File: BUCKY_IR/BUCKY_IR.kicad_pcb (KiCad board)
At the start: 2 copper layers, 189.9 x 157.6 mm, 37 parts, among them J1 SERIAL_CONN, J2 CAN_CONN_UP, J3 CAN_CONN_DOWN, U1 TSSP96038TR, U10 TSSP96038TR, U11 TSSP96038TR, U12 TSSP96038TR, U13 TSSP96038TR, U14 TSSP96038TR, U15 TSSP96038TR, U16 TSSP96038TR, U17 SN65HVD230, U18 ESP32-WROOM-32U, U19 AMS1117-5.0, U2 TSSP96038TR, U3 TSSP96038TR, U4 TSSP96038TR, U5 TSSP96038TR, U6 TSSP96038TR, U7 TSSP96038TR, U8 TSSP96038TR, U9 TSSP96038TR

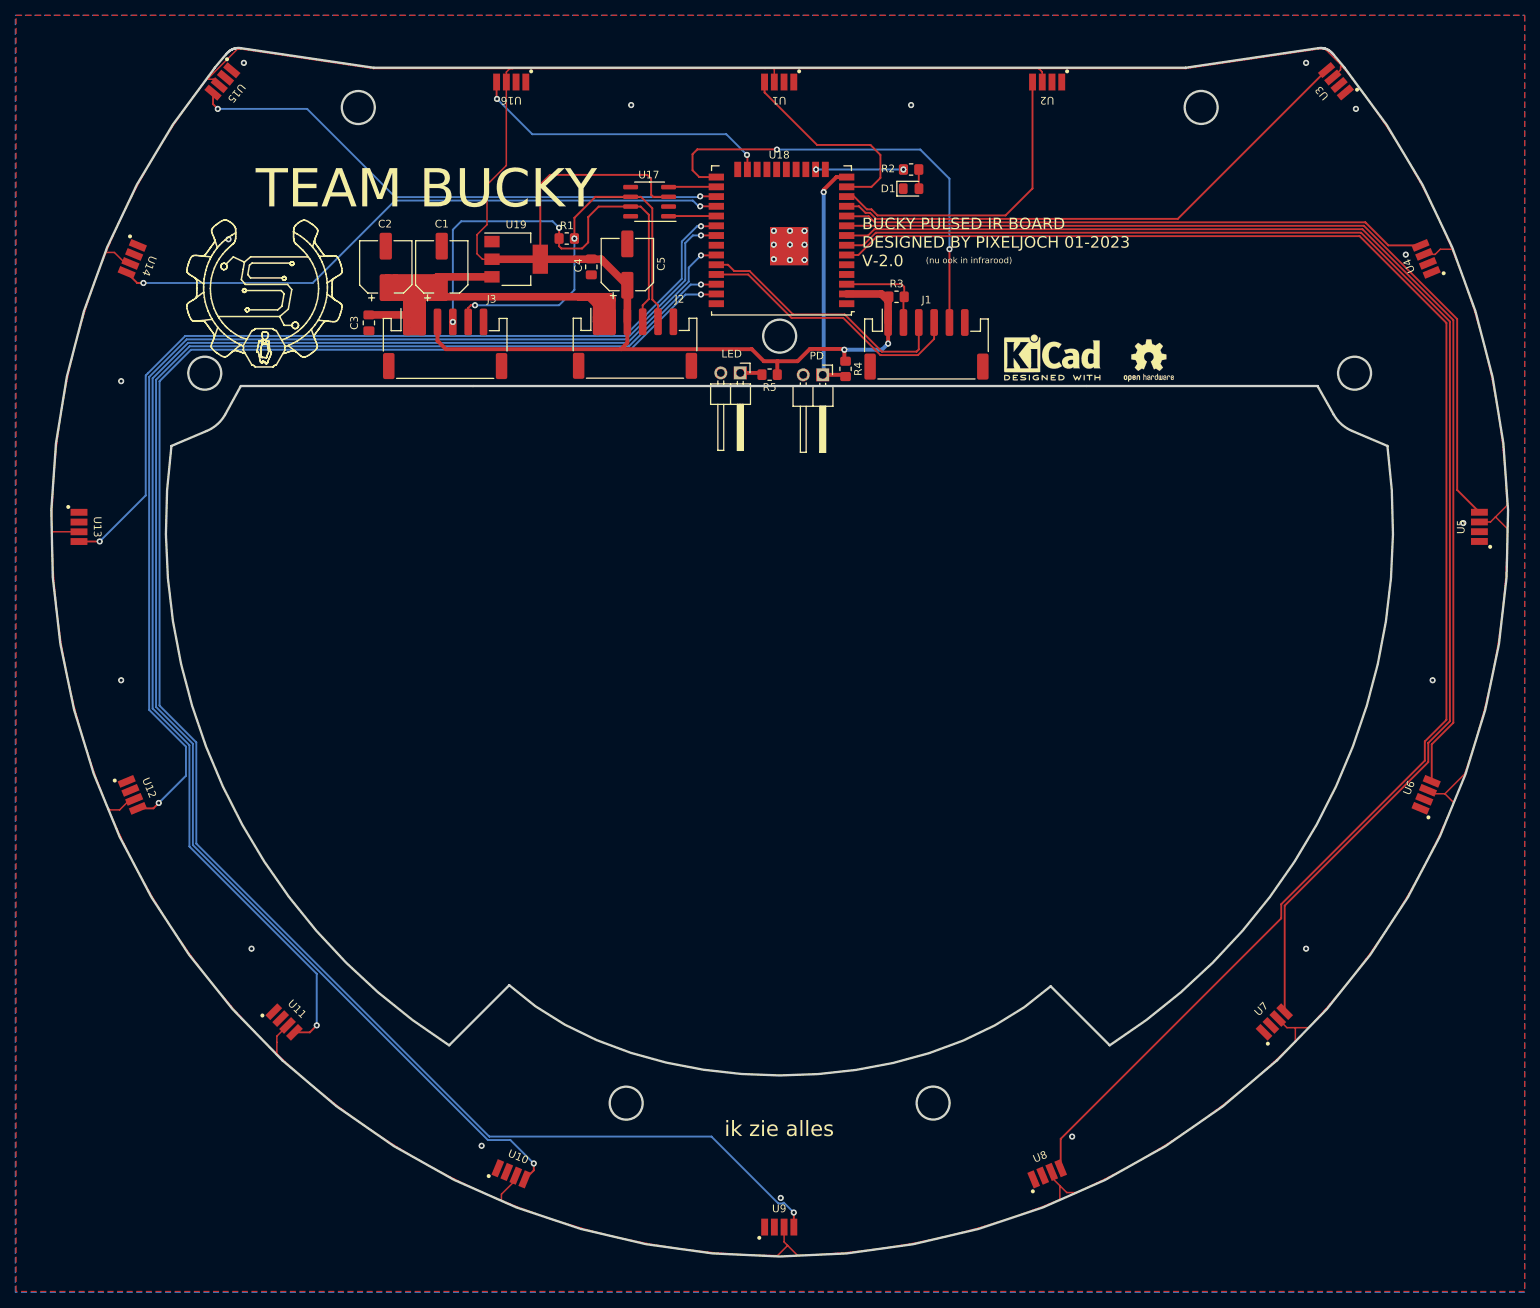
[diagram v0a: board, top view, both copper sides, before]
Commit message: chore: start on schematics
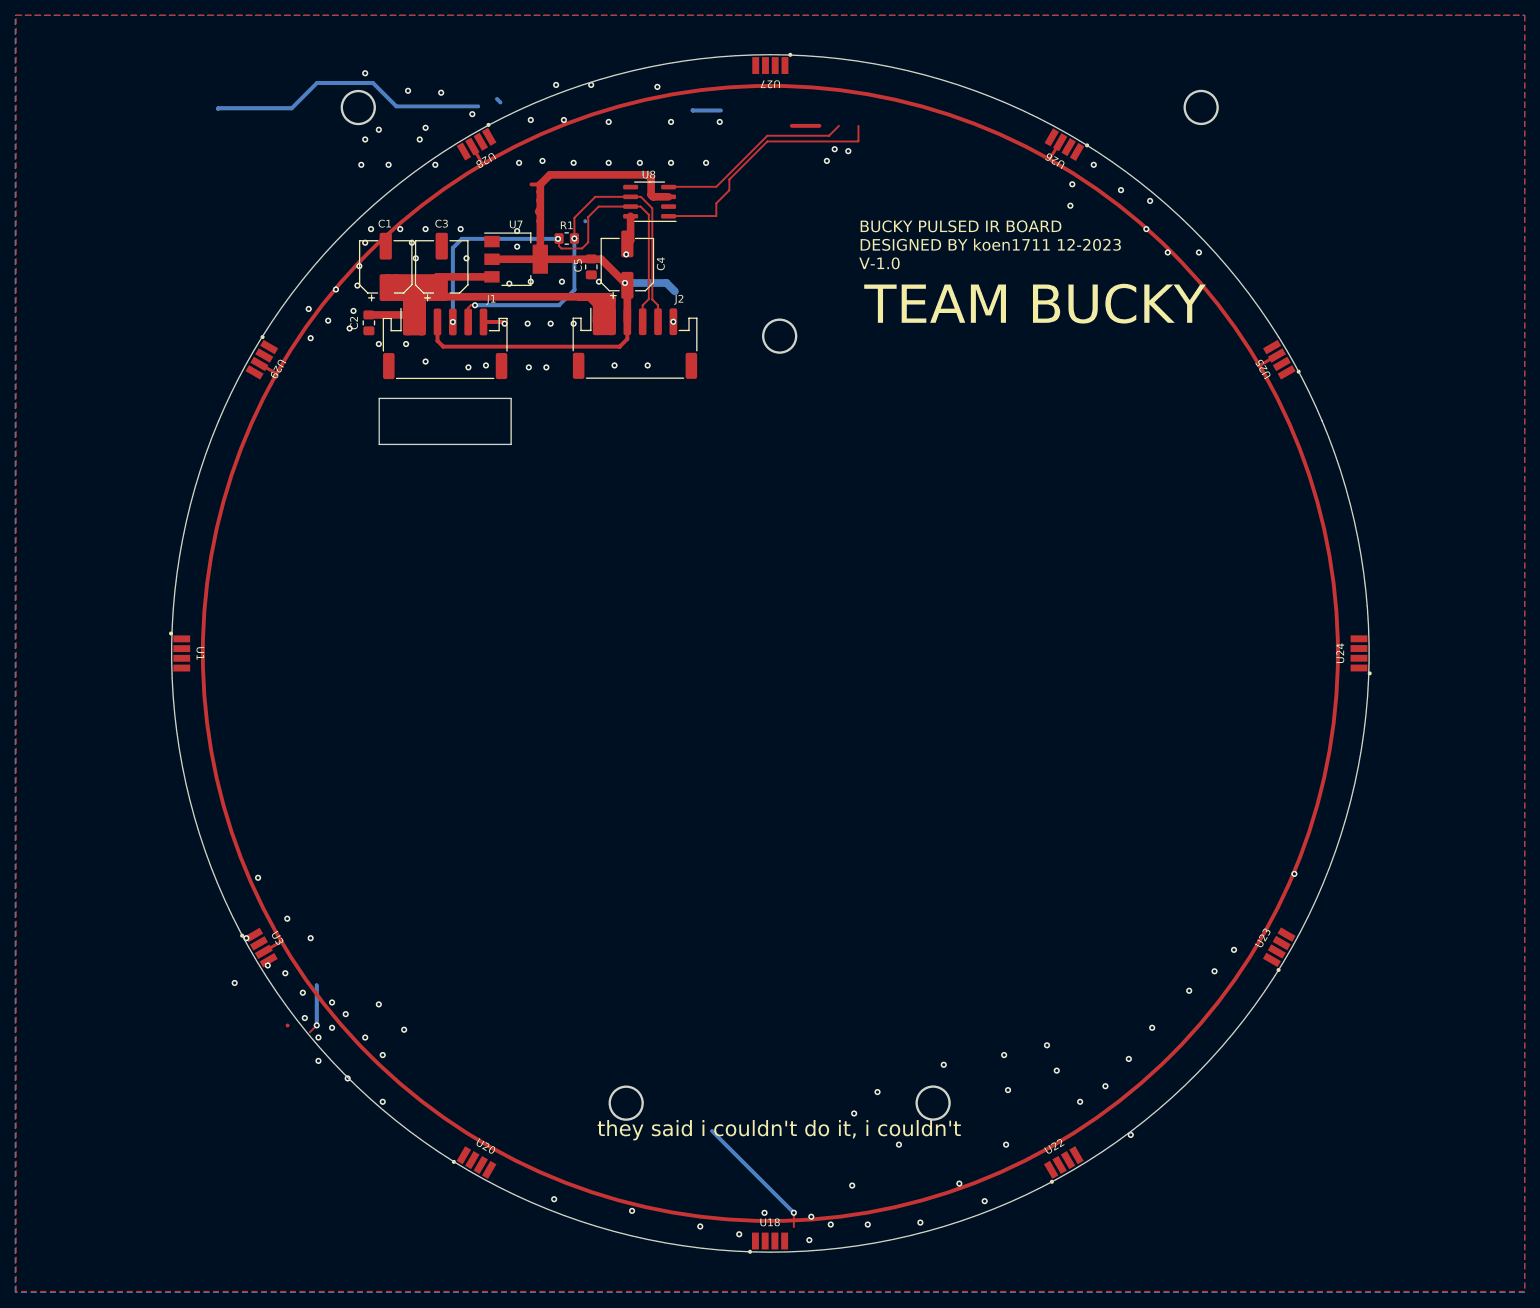
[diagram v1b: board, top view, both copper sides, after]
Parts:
- removed D1: LED, LED_SMD:LED_0805_2012Metric_Pad1.15x1.40mm_HandSolder
- removed the J1 at (141.0, 57.7)
- removed LED: LED, Connector_PinHeader_2.54mm:PinHeader_1x02_P2.54mm_Horizontal
- removed PD: PHOTODIODE, Connector_PinHeader_2.54mm:PinHeader_1x02_P2.54mm_Horizontal
- removed R2, R5: 120R, Resistor_SMD:R_0805_2012Metric_Pad1.20x1.40mm_HandSolder
- removed R3, R4: 10k, Resistor_SMD:R_0805_2012Metric_Pad1.20x1.40mm_HandSolder
- removed REF**: KiCad-Logo2_5mm_SilkScreen, Symbol:KiCad-Logo2_5mm_SilkScreen
- removed REF**: OSHW-Logo2_7.3x6mm_SilkScreen, Symbol:OSHW-Logo2_7.3x6mm_SilkScreen
- removed U10, U11, U12, U13, U14, U15, U16, U2, U4, U5, U6: TSSP96038TR, BUCKY_IR:TSSP96038
- removed the U18 at (122.1, 44.1)
- removed the U7 at (186.4, 146.1)
- removed the U8 at (156.7, 165.9)
- added U20: TSSP96038TR, BUCKY_IR:TSSP96038, F.Cu at (82.3, 164.4)
- added U22: TSSP96038TR, BUCKY_IR:TSSP96038, F.Cu at (158.9, 164.4)
- added U23: TSSP96038TR, BUCKY_IR:TSSP96038, F.Cu at (187.0, 136.3)
- added U24: TSSP96038TR, BUCKY_IR:TSSP96038, F.Cu at (197.4, 98.0)
- added U25: TSSP96038TR, BUCKY_IR:TSSP96038, F.Cu at (187.0, 59.7)
- added U26: TSSP96038TR, BUCKY_IR:TSSP96038, F.Cu at (159.0, 31.7)
- added U27: TSSP96038TR, BUCKY_IR:TSSP96038, F.Cu at (120.7, 21.4)
- added U28: TSSP96038TR, BUCKY_IR:TSSP96038, F.Cu at (82.3, 31.6)
- added U29: TSSP96038TR, BUCKY_IR:TSSP96038, F.Cu at (54.4, 59.7)
- moved U3 180.0 mm to (54.3, 136.3), turned to -60 degrees
- moved U1 107.8 mm to (43.9, 98.0), turned to -90 degrees
- moved U18 2.18 mm to (120.6, 174.6)
- renumbered C2 to C1, C3 to C2, C1 to C3, C5 to C4, C4 to C5, J3 to J1, U9 to U18, U19 to U7, U17 to U8
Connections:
- U3 pad 4: /IR_3 -> /IR_1
- U8 pad 8: unconnected-(U17-Pad8) -> GND
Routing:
- net +3V3: track 792.2 -> 92.7 mm, vias 2 -> 1
- net /IR_9: track 239.4 -> 17.0 mm, vias 2 -> 1
- net /IR_8: track 215.0 -> 0.00 mm
- net /IR_10: track 205.1 -> 0.00 mm, vias 2 -> 0
- net /IR_7: track 183.0 -> 0.00 mm
- net /IR_11: track 177.7 -> 6.53 mm, vias 2 -> 1
- net /IR_12: track 146.5 -> 0.00 mm, vias 2 -> 0
- net /IR_6: track 145.7 -> 0.00 mm
- net /IR_13: track 112.2 -> 0.00 mm, vias 2 -> 0
- net /IR_5: track 111.0 -> 0.00 mm
- net /IR_14: track 82.2 -> 0.00 mm, vias 2 -> 0
- net /IR_4: track 76.4 -> 0.00 mm
- net /IR_3: track 71.3 -> 0.00 mm
- net /IO_0: track 59.7 -> 0.00 mm, vias 2 -> 0
- net /IR_2: track 40.6 -> 0.00 mm
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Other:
- board size 189.9 x 157.6 mm -> 156.1 x 156.1 mm
- board text added: "BUCKY PULSED IR BOARD DESIGNED BY koen1711 12-2023 V-1.0"
- board text added: "they said i couldn't do it, i couldn't"
- board text removed: "(nu ook in infrarood)"
- board text removed: "BUCKY PULSED IR BOARD DESIGNED BY PIXELJOCH 01-2023 V-2.0"
- board text removed: "ik zie alles"
